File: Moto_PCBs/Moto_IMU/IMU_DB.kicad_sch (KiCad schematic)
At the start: 27 parts, among them J1 POWER IN, J2 CANBUS, J3 Conn_01x05_Pin 61300511121, U1 STM32F103C8Tx, U2 IAM-20680HP, U3 SN65HVD230

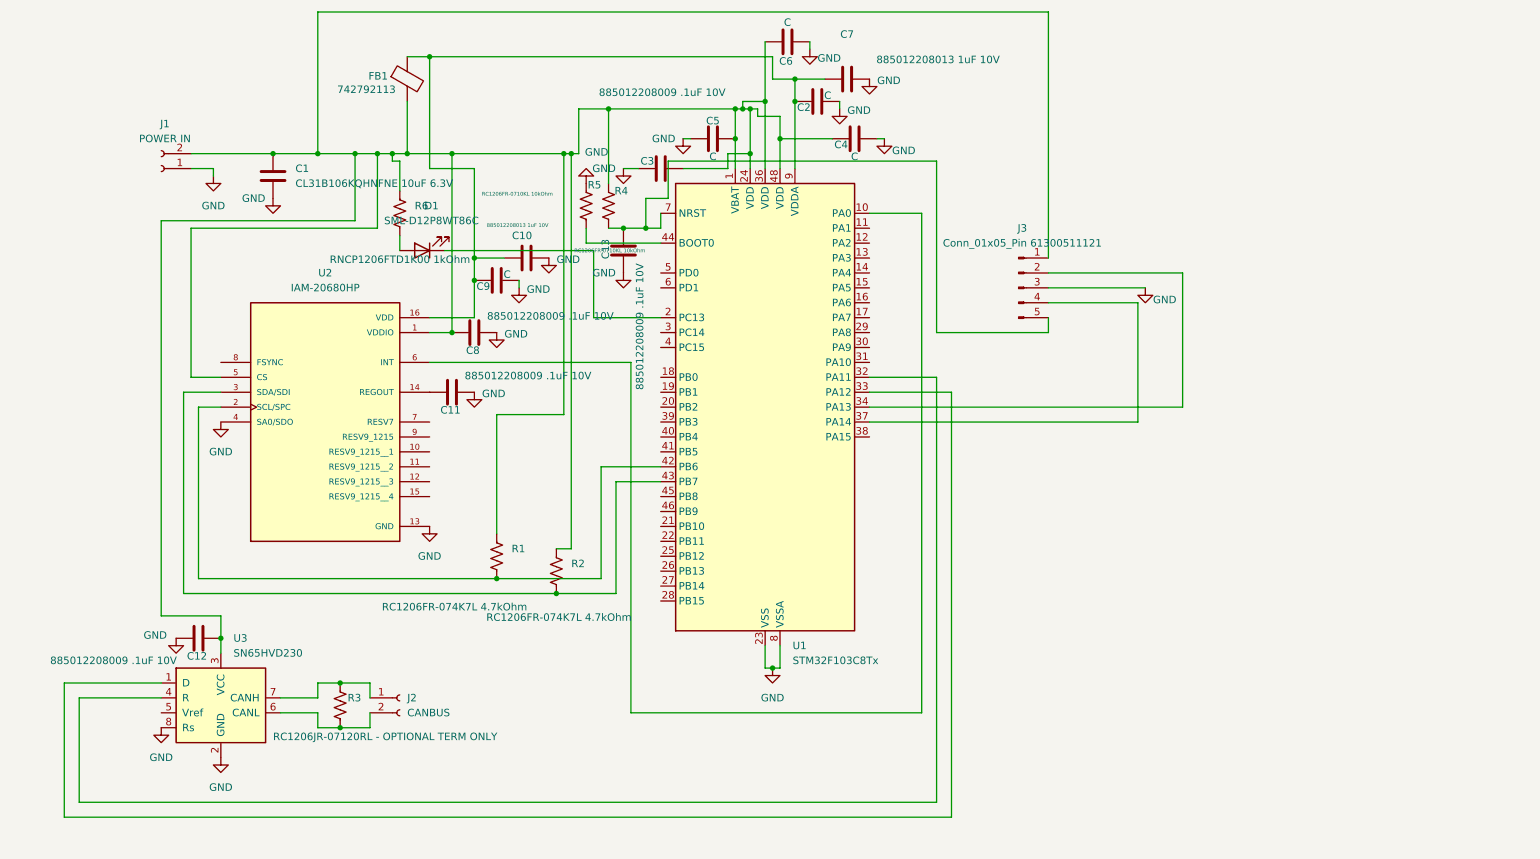
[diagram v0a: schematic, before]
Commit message: Add files via upload
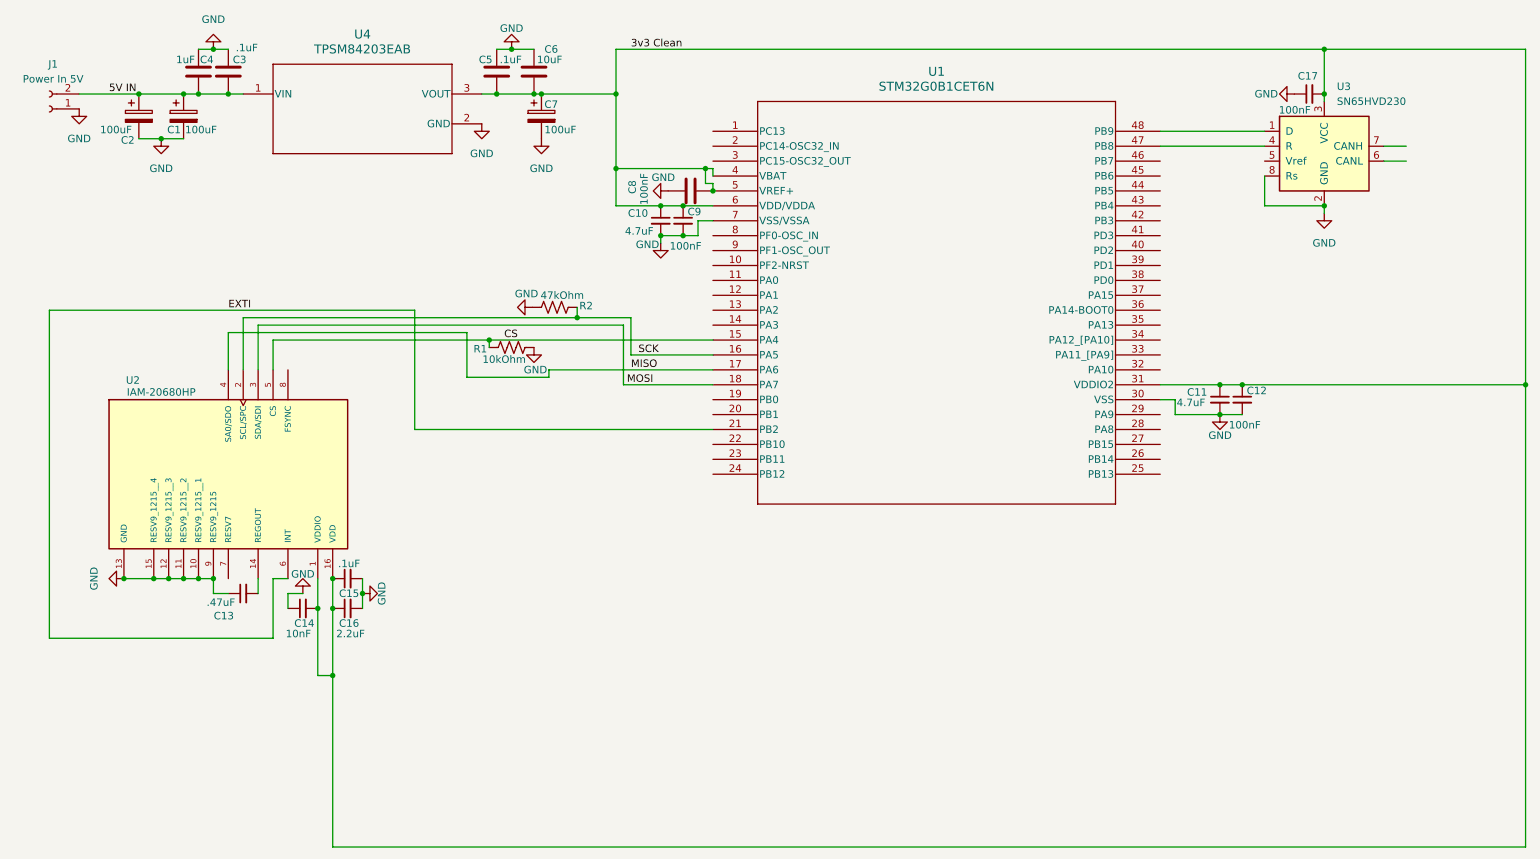
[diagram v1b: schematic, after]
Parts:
- removed C1: CL31B106KQHNFNE 10uF 6.3V, Capacitor_SMD:C_1206_3216Metric_Pad1.33x1.80mm_HandSolder, symbol Device:C
- removed C10, C7: 885012208013 1uF 10V, Capacitor_SMD:C_1206_3216Metric_Pad1.33x1.80mm_HandSolder, symbol Device:C
- removed C11, C12, C13: 885012208009 .1uF 10V, Capacitor_SMD:C_1206_3216Metric_Pad1.33x1.80mm_HandSolder, symbol Device:C
- removed C2, C9: C, Capacitor_SMD:C_1206_3216Metric_Pad1.33x1.80mm_HandSolder, symbol Device:C
- removed D1: SML-D12P8WT86C, LED_SMD:LED_0603_1608Metric_Pad1.05x0.95mm_HandSolder, symbol Device:LED
- removed FB1: 742792113, Inductor_SMD:L_1206_3216Metric_Pad1.42x1.75mm_HandSolder, symbol Device:FerriteBead
- removed J2: CANBUS, Connector_Molex:Molex_Micro-Fit_3.0_43650-0200_1x02_P3.00mm_Horizontal, symbol Connector:Conn_01x02_Socket
- removed J3: Conn_01x05_Pin 61300511121, Connector_PinHeader_2.54mm:PinHeader_1x05_P2.54mm_Vertical, symbol Connector:Conn_01x05_Pin
- removed R3: RC1206JR-07120RL - OPTIONAL TERM ONLY, Resistor_SMD:R_1206_3216Metric_Pad1.30x1.75mm_HandSolder, symbol Device:R_US
- removed R4, R5: RC1206FR-0710KL 10kOhm, Resistor_SMD:R_1206_3216Metric_Pad1.30x1.75mm_HandSolder, symbol Device:R_US
- removed R6: RNCP1206FTD1K00 1kOhm, Resistor_SMD:R_1206_3216Metric_Pad1.30x1.75mm_HandSolder, symbol Device:R_US
- removed U1: STM32F103C8Tx, Package_QFP:LQFP-48_7x7mm_P0.5mm, symbol MCU_ST_STM32F1:STM32F103C8Tx
- added C1, C2, C7: 100uF, Capacitor_THT:CP_Radial_D5.0mm_P2.50mm, symbol Device:C_Polarized
- added C10, C11: 4.7uF, Capacitor_SMD:C_0805_2012Metric_Pad1.18x1.45mm_HandSolder, symbol Device:C_Small
- added C12, C17, C9: 100nF, Capacitor_SMD:C_0805_2012Metric_Pad1.18x1.45mm_HandSolder, symbol Device:C_Small
- added C13: .47uF, Capacitor_SMD:C_0805_2012Metric_Pad1.18x1.45mm_HandSolder, symbol Device:C_Small
- added C14: 10nF, Capacitor_SMD:C_0805_2012Metric_Pad1.18x1.45mm_HandSolder, symbol Device:C_Small
- added C15: .1uF, Capacitor_SMD:C_0805_2012Metric_Pad1.18x1.45mm_HandSolder, symbol Device:C_Small
- added C16: 2.2uF, Capacitor_SMD:C_0805_2012Metric_Pad1.18x1.45mm_HandSolder, symbol Device:C_Small
- added U1: STM32G0B1CET6N, LQFP48_STM, symbol 2026-07-01_13-54-37:STM32G0B1CET6N
- added U4: TPSM84203EAB, TPSM84203EAB:EAB0003A, symbol TPSM84203EAB:TPSM84203EAB
- C3: value 885012208009 .1uF 10V -> .1uF; footprint Capacitor_SMD:C_1206_3216Metric_Pad1.33x1.80mm_HandSolder -> Capacitor_SMD:C_0805_2012Metric_Pad1.18x1.45mm_HandSolder
- C4: value C -> 1uF; footprint Capacitor_SMD:C_1206_3216Metric_Pad1.33x1.80mm_HandSolder -> Capacitor_SMD:C_0805_2012Metric_Pad1.18x1.45mm_HandSolder
- C5: value C -> .1uF; footprint Capacitor_SMD:C_1206_3216Metric_Pad1.33x1.80mm_HandSolder -> Capacitor_SMD:C_0805_2012Metric_Pad1.18x1.45mm_HandSolder
- C6: value C -> 10uF; footprint Capacitor_SMD:C_1206_3216Metric_Pad1.33x1.80mm_HandSolder -> Capacitor_SMD:C_0805_2012Metric_Pad1.18x1.45mm_HandSolder
- C8: value 885012208009 .1uF 10V -> 100nF; footprint Capacitor_SMD:C_1206_3216Metric_Pad1.33x1.80mm_HandSolder -> Capacitor_SMD:C_0805_2012Metric_Pad1.18x1.45mm_HandSolder
- J1: value POWER IN -> Power In 5V; footprint Connector_Molex:Molex_Micro-Fit_3.0_43650-0200_1x02_P3.00mm_Horizontal -> 0436500201:CONN_SD-43650-001_02_MOL
- R1: value RC1206FR-074K7L 4.7kOhm -> 10kOhm; footprint Resistor_SMD:R_1206_3216Metric_Pad1.30x1.75mm_HandSolder -> Resistor_SMD:R_0805_2012Metric_Pad1.20x1.40mm_HandSolder
- R2: value RC1206FR-074K7L 4.7kOhm -> 47kOhm; footprint Resistor_SMD:R_1206_3216Metric_Pad1.30x1.75mm_HandSolder -> Resistor_SMD:R_0805_2012Metric_Pad1.20x1.40mm_HandSolder
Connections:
- net GND: now also C4.1, C6.1, R1.2, R2.2, U2.10 (RESV9_1215__1), U2.11 (RESV9_1215__2), U2.12 (RESV9_1215__3), U2.15 (RESV9_1215__4), U2.9 (RESV9_1215), C1.2, C10.2, C11.2, C12.2, C13.1, C14.1, C15.2, C16.2, C17.1, C2.2, C7.2, C9.2, U1.30 (VSS), U1.7 (VSS/VSSA), U4.2 (GND); no longer C4.2, C6.2, U2.4 (SA0/SDO)
- net 3v3 Clean: now reaches U2.16 (VDD)
- net 3v3 Clean: now also C5.2, C6.2, C8.2, U2.1 (VDDIO), U3.3 (VCC), C10.1, C11.1, C12.1, C14.2, C15.1, C16.1, C17.2, C7.1, C9.1, U1.31 (VDDIO2), U1.4 (VBAT), U1.5 (VREF+), U1.6 (VDD/VDDA), U4.3 (VOUT)
- net at U3.1 (D): now also U1.48 (PB9)
- net at U3.4 (R): now also U1.47 (PB8)
- net at U2.14 (REGOUT): now also C13.2
- net MOSI: now reaches U2.3 (SDA/SDI)
- net MOSI: now also U1.18 (PA7); no longer R2.2
- net SCK: now reaches U2.2 (SCL/SPC)
- net SCK: now also R2.1, U1.16 (PA5); no longer R1.2
- net EXTI: now reaches U2.6 (INT)
- net EXTI: now also U1.21 (PB2)
- new net 5V IN: C1.1, C2.1, C3.2, C4.2, J1.2 (Pin_2), U4.1 (VIN)
- new net CS: R1.1, U1.15 (PA4), U2.5 (CS)
- new net MISO: U1.17 (PA6), U2.4 (SA0/SDO)
